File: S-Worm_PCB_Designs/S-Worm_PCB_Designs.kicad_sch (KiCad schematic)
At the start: 60 parts

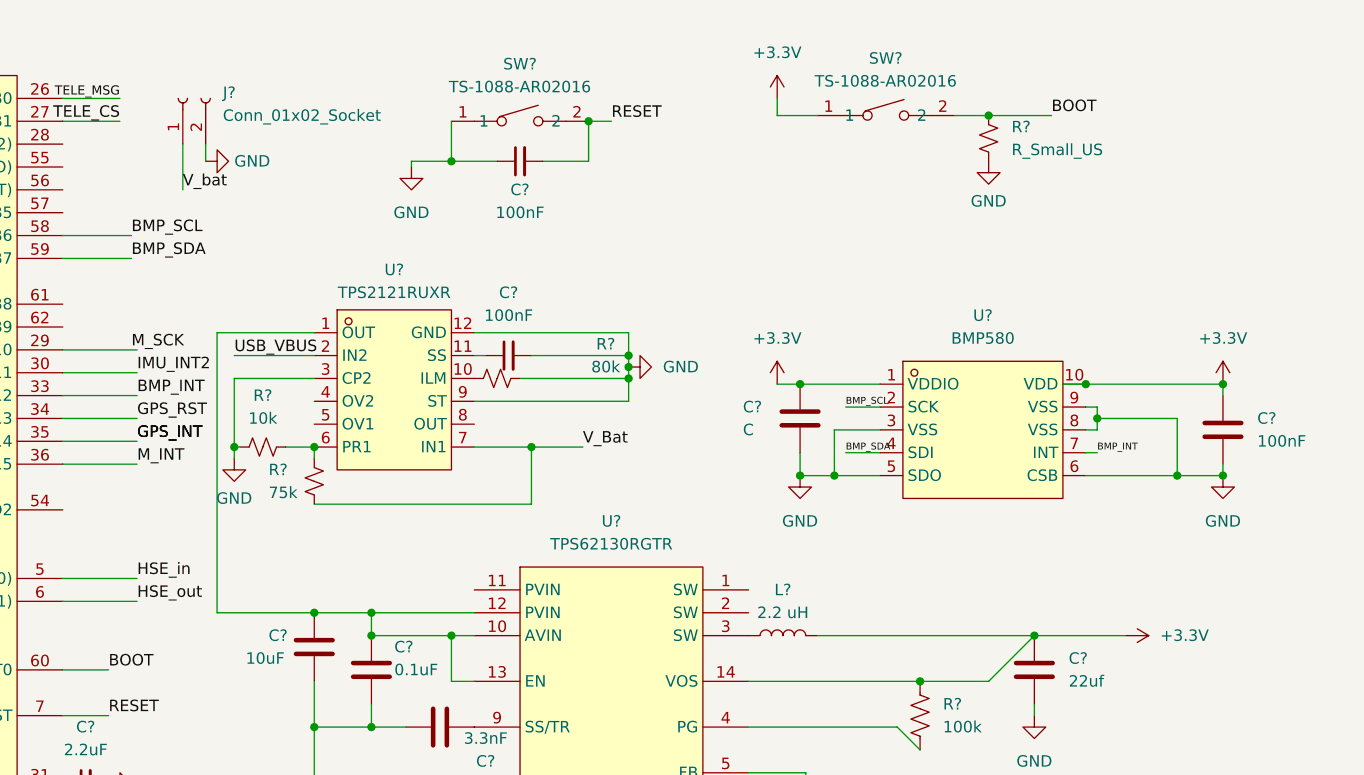
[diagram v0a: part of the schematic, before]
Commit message: adc aaa
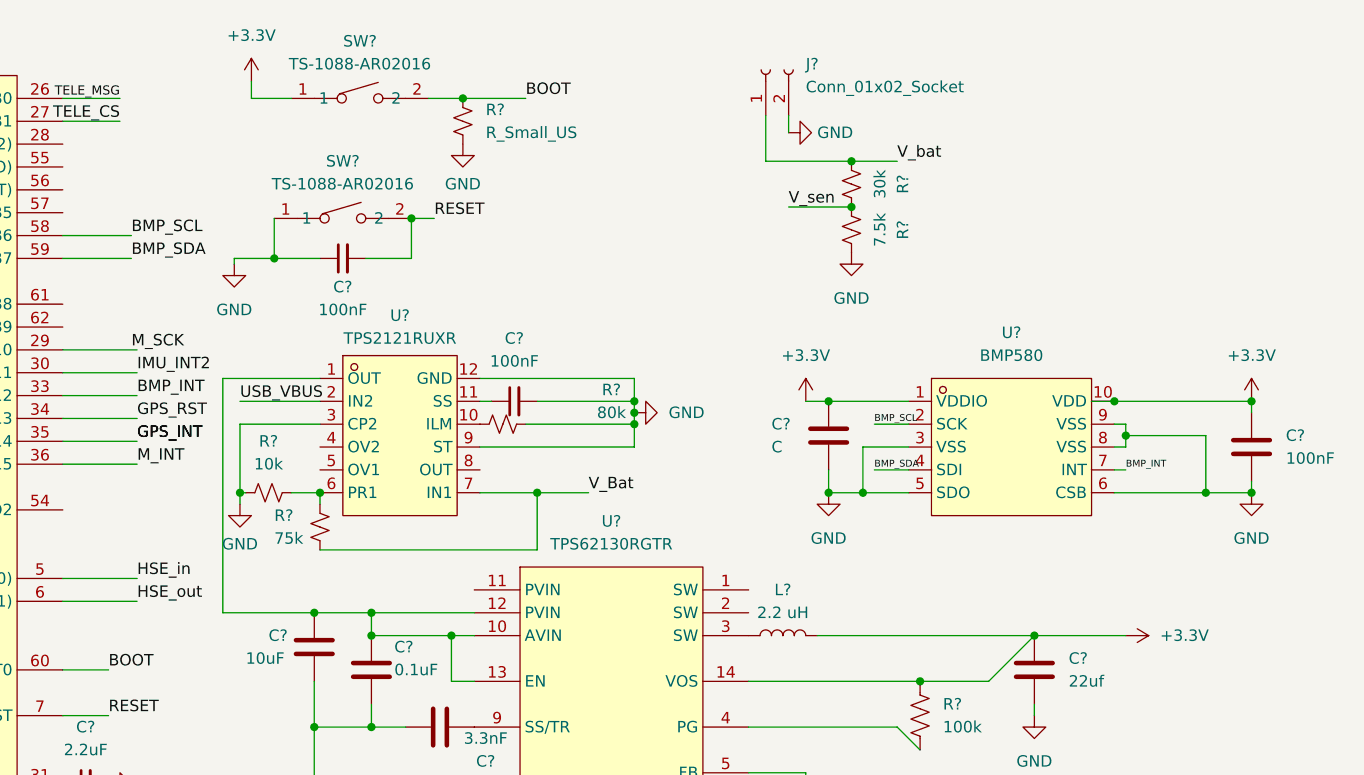
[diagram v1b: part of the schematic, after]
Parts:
- added R?: 30k, symbol Device:R_Small_US
- added R?: 7.5k, symbol Device:R_Small_US
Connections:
- net GND: now also R?.2
- net V_bat: now also R?.1
- new net V_sen: R?.1, R?.2
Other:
- moved on the sheet: C?, J?, R?, SW?, U?
